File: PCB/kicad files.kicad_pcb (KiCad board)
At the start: 2 copper layers, 93 x 90.5 mm, 35 parts, among them J2 Conn_01x04_Pin, SW1 SW_Push_45deg, SW10 RotaryEncoder_Switch, SW2 SW_Push_45deg, SW3 SW_Push_45deg, SW4 SW_Push_45deg, SW5 SW_Push_45deg, SW6 SW_Push_45deg, SW7 SW_Push_45deg, SW8 SW_Push_45deg, SW9 SW_Push_45deg, U2 MOUDLE-SEEEDUINO-XIAO

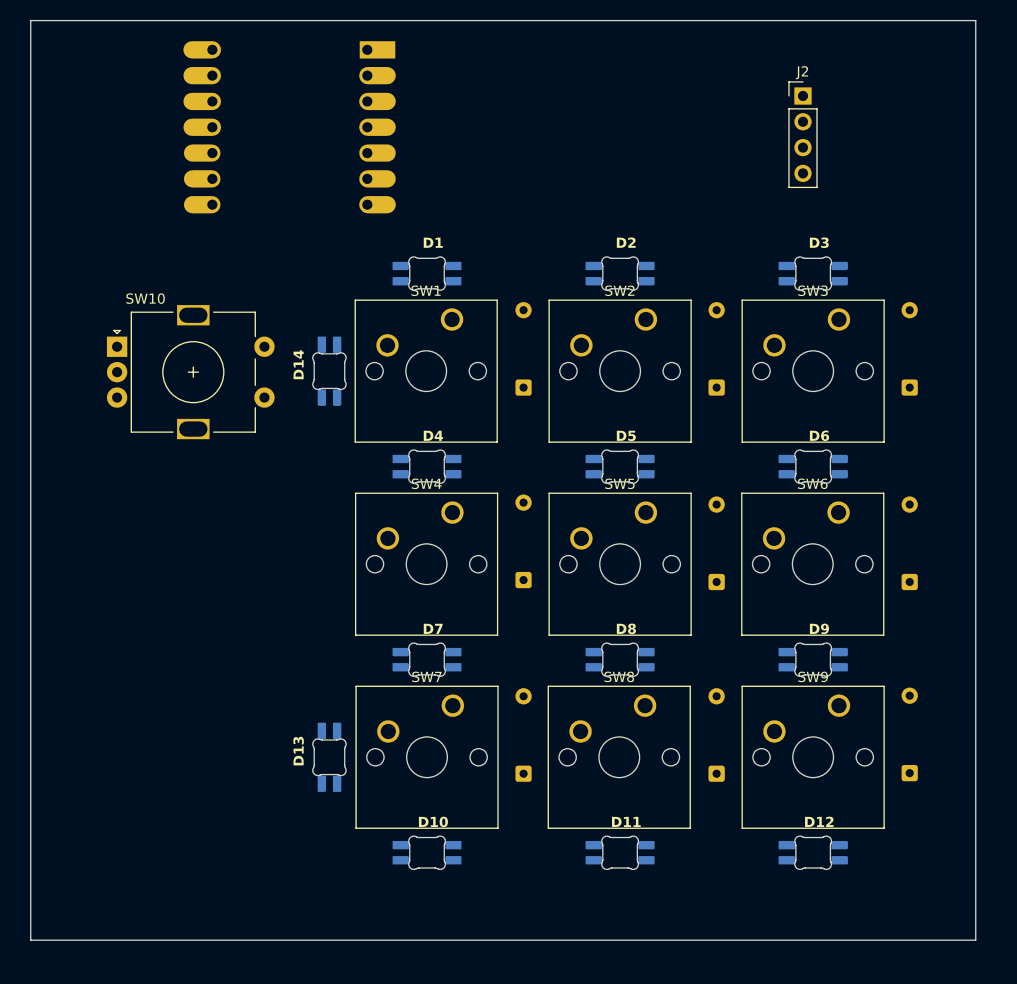
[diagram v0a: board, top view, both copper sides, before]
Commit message: pcb finally done with 64 fucking errorss
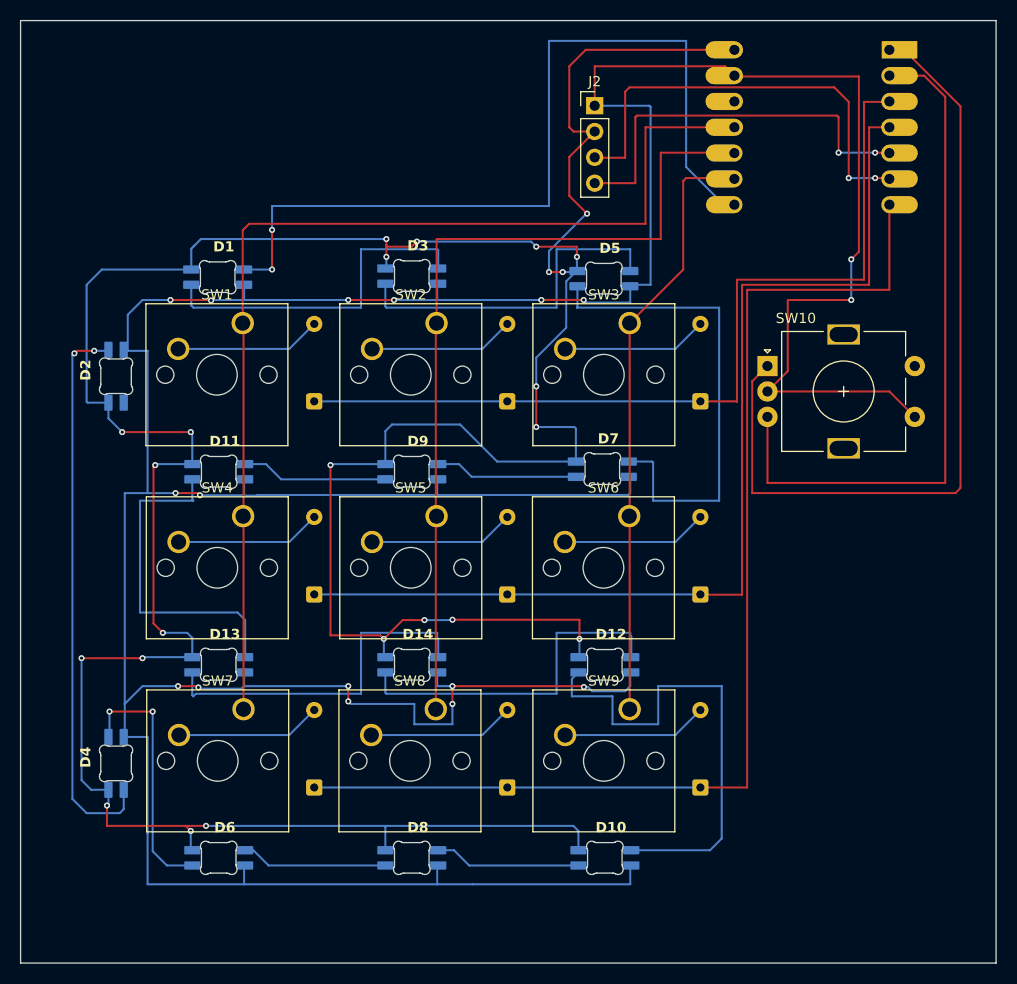
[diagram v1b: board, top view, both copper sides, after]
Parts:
- moved D6 70.0 mm to (98.5, 123.5)
- moved SW10 64.0 mm to (152.5, 75.0)
- moved D33 58.6 mm to (107.9, 116.5)
- moved D27 58.6 mm to (107.9, 78.5)
- moved D30 58.6 mm to (107.9, 97.5)
- moved D11 54.5 mm to (98.5, 85.5)
- moved U2 51.4 mm to (156.9, 51.5)
- moved D2 50.5 mm to (88.5, 76.0), turned to 90 degrees
- moved D9 43.6 mm to (117.5, 85.5)
- moved D4 42.2 mm to (88.5, 114.1), turned to 90 degrees
- moved D3 39.5 mm to (117.5, 66.2)
- moved D14 30.1 mm to (117.5, 104.5), turned to 0 degrees
- moved D8 28.3 mm to (117.5, 123.5)
- moved D12 27.6 mm to (136.5, 104.5)
- moved D7 25.5 mm to (136.2, 85.2)
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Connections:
- U2 pad 10: Column 1 -> column 1
- U2 pad 11: Column 0 -> column 0
- U2 pad 9: Column 2 -> column 2
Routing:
- net GND: track 0.00 -> 397.5 mm, vias 0 -> 17
- net +5V: track 0.00 -> 340.4 mm, vias 0 -> 24
- net Row 2: track 0.00 -> 114.0 mm
- net column 0: track 0.00 -> 105.3 mm
- net Row 1: track 0.00 -> 102.6 mm
- net Row 0: track 0.00 -> 86.1 mm
- net LED Data: track 0.00 -> 84.7 mm, vias 0 -> 2
- net column 1: track 0.00 -> 84.1 mm
- net ENC_A: track 0.00 -> 80.7 mm
- net ENC_B: track 0.00 -> 68.9 mm
- net column 2: track 0.00 -> 59.4 mm
- net Net-(D2-DIN): track 0.00 -> 55.1 mm, vias 0 -> 2
- net Net-(D10-DIN): track 0.00 -> 48.2 mm
- net Net-(D5-DOUT): track 0.00 -> 47.8 mm
- net SCL: track 0.00 -> 43.8 mm, vias 0 -> 2
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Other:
- board size 93 x 90.5 mm -> 96 x 92.8 mm
